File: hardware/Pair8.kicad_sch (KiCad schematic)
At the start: 10 parts, among them IC8 TPS2HCS08AQPWPRQ1, J11 Conn_01x02, J19 Conn_01x02

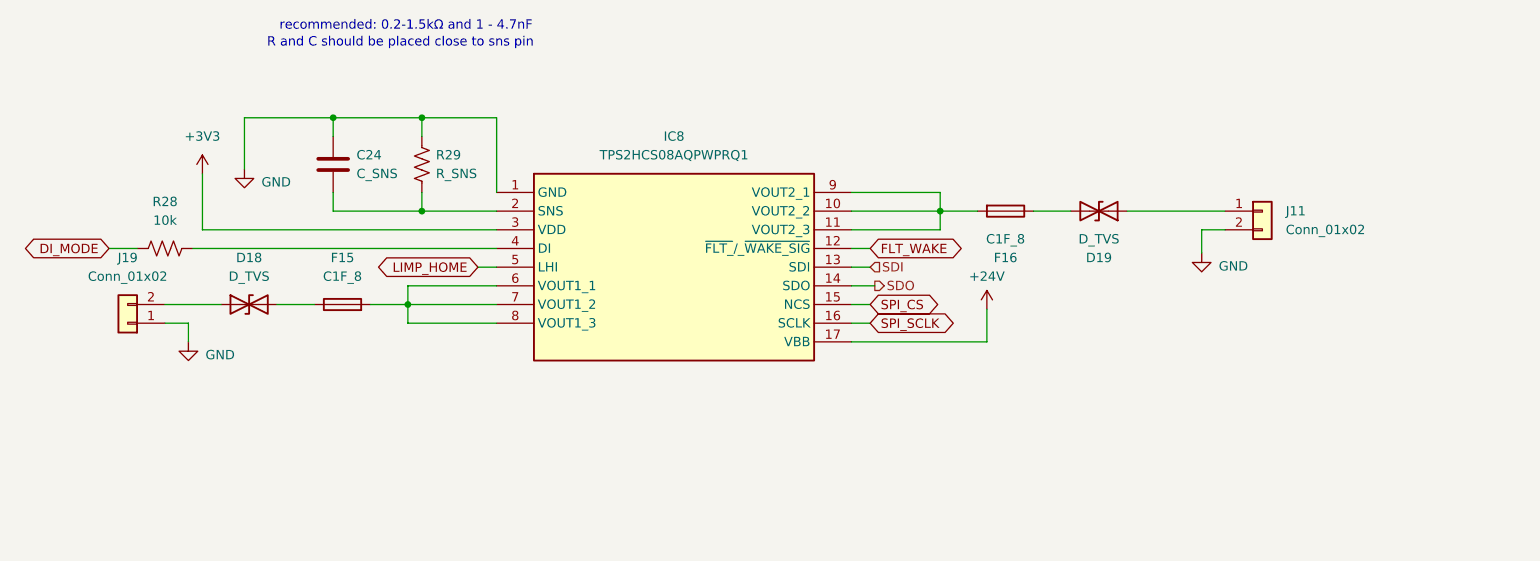
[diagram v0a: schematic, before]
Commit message: aesthetic added
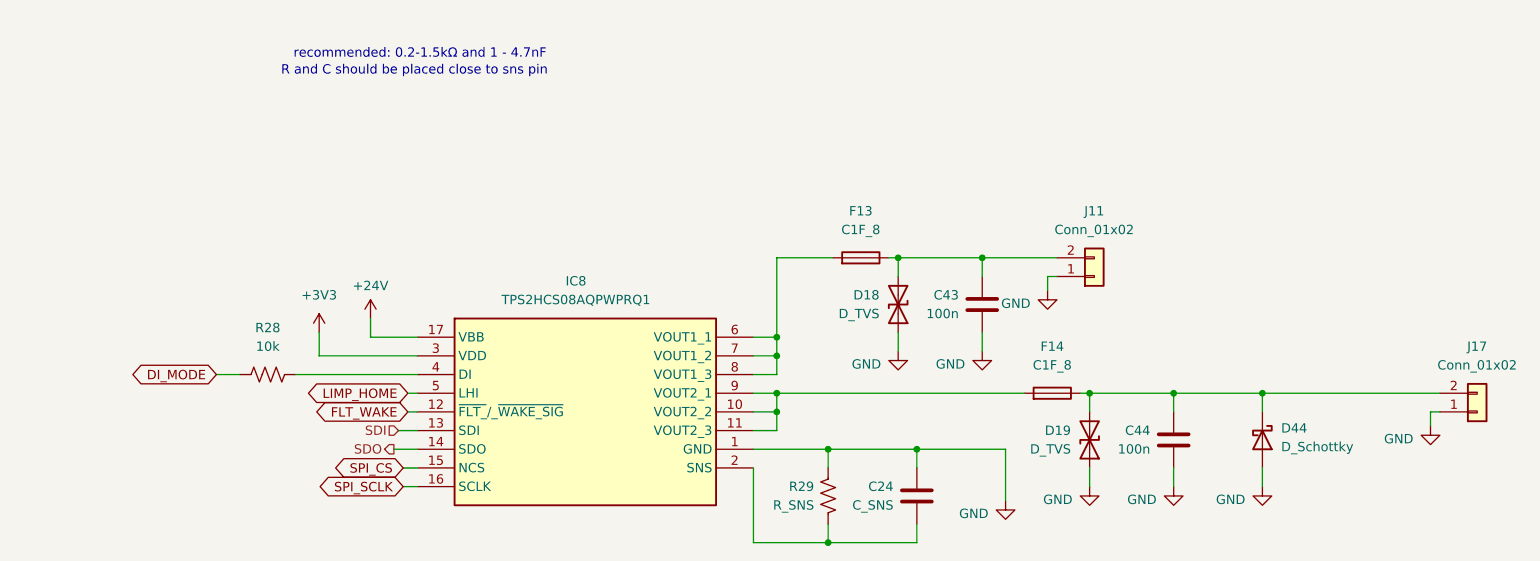
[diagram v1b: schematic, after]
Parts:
- removed F15, F16: C1F_8, Fuse:Fuse_1206_3216Metric, symbol PowerDistributionUnitLib:C1F_8
- removed J19: Conn_01x02, symbol Connector_Generic:Conn_01x02
- added C43, C44: 100n, symbol Device:C
- added D44: D_Schottky, symbol Device:D_Schottky
- added F13, F14: C1F_8, Fuse:Fuse_1206_3216Metric, symbol PowerDistributionUnitLib:C1F_8
- added J17: Conn_01x02, symbol Connector_Generic:Conn_01x02
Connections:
- net GND: now also D18.1 (A1), D19.1 (A1), J11.1 (Pin_1), C43.1, C44.1, D44.2 (A), J17.1 (Pin_1); no longer J11.2 (Pin_2)
- net at D19.2 (A2): now also C44.2, D44.1 (K), F14.1, J17.2 (Pin_2)
- net at IC8.10 (VOUT2_2), IC8.11 (VOUT2_3), IC8.9 (VOUT2_1): now also F14.2
- net at IC8.6 (VOUT1_1), IC8.7 (VOUT1_2), IC8.8 (VOUT1_3): now also F13.2
- net at D18.2 (A2): now also J11.2 (Pin_2), C43.2, F13.1
